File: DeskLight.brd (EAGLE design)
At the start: 44.5 x 58.4 mm, 39 parts, among them IC1 REG1117, J1 Würth Elektronik SD Connector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, T1 MMBT2222, T2 MMBT2222, T3 MJD122, T4 MJD122, T5 MJD122, U1 ESP32-WROOM-32D, U2 CH340C

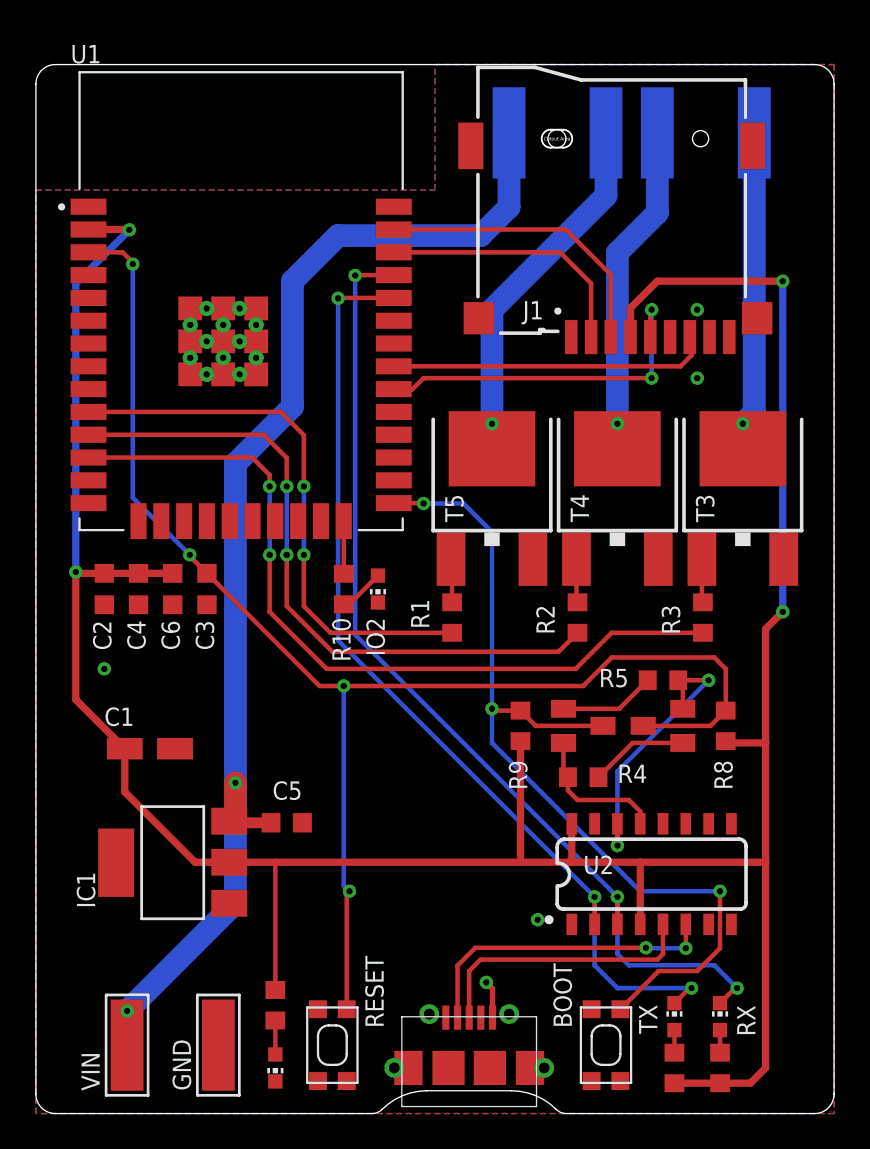
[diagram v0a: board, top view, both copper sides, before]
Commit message: .
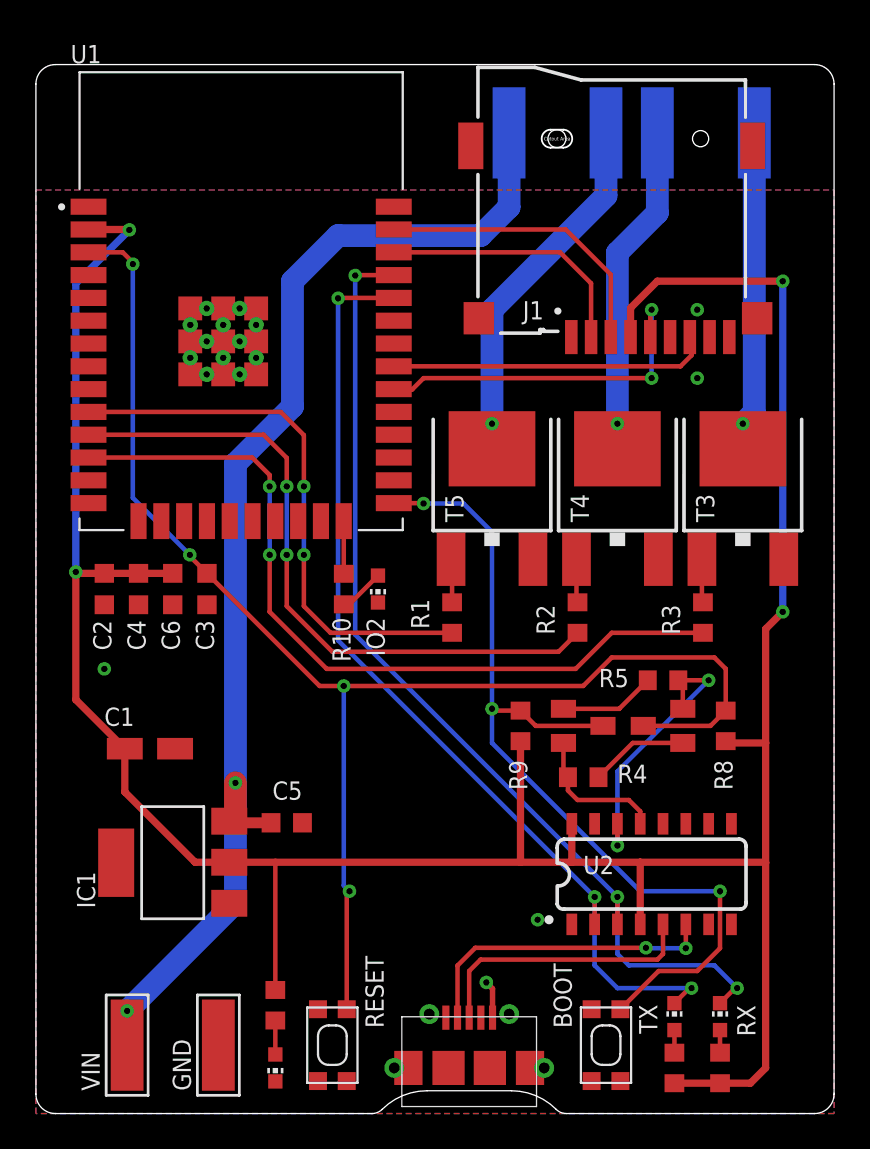
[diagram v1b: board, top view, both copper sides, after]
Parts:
- IC1: device burr-brown:SOT223 -> burr-brown_:SOT223
